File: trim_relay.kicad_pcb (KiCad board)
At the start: 2 copper layers, 75 x 75 mm, 45 parts, among them J1 Conn_01x01, J10 Conn_01x01, J11 Conn_01x01, J2 Conn_01x01, J3 Conn_01x01, J4 Conn_01x01, J5 Conn_01x01, J6 Conn_01x01, J7 Conn_01x01, J8 Conn_01x01, J9 Conn_01x01, K1 G5LE, K2 G5LE, K3 G5LE, K4 G5LE, K5 G5LE, Q1 2N3906, Q2 2N3906, Q3 2N3906, Q4 2N3906, Q5 2N3906, U1 LM317L_TO92

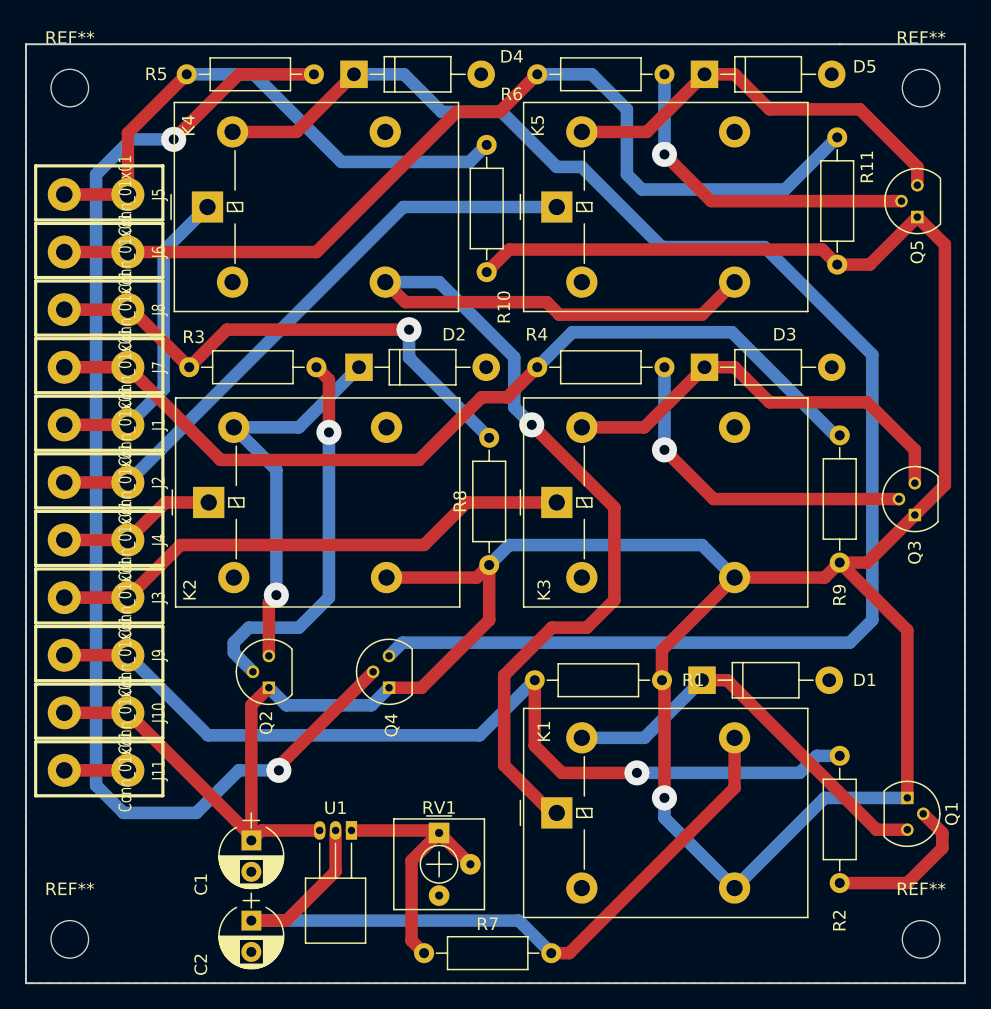
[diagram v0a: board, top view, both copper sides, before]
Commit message: Fixed layout
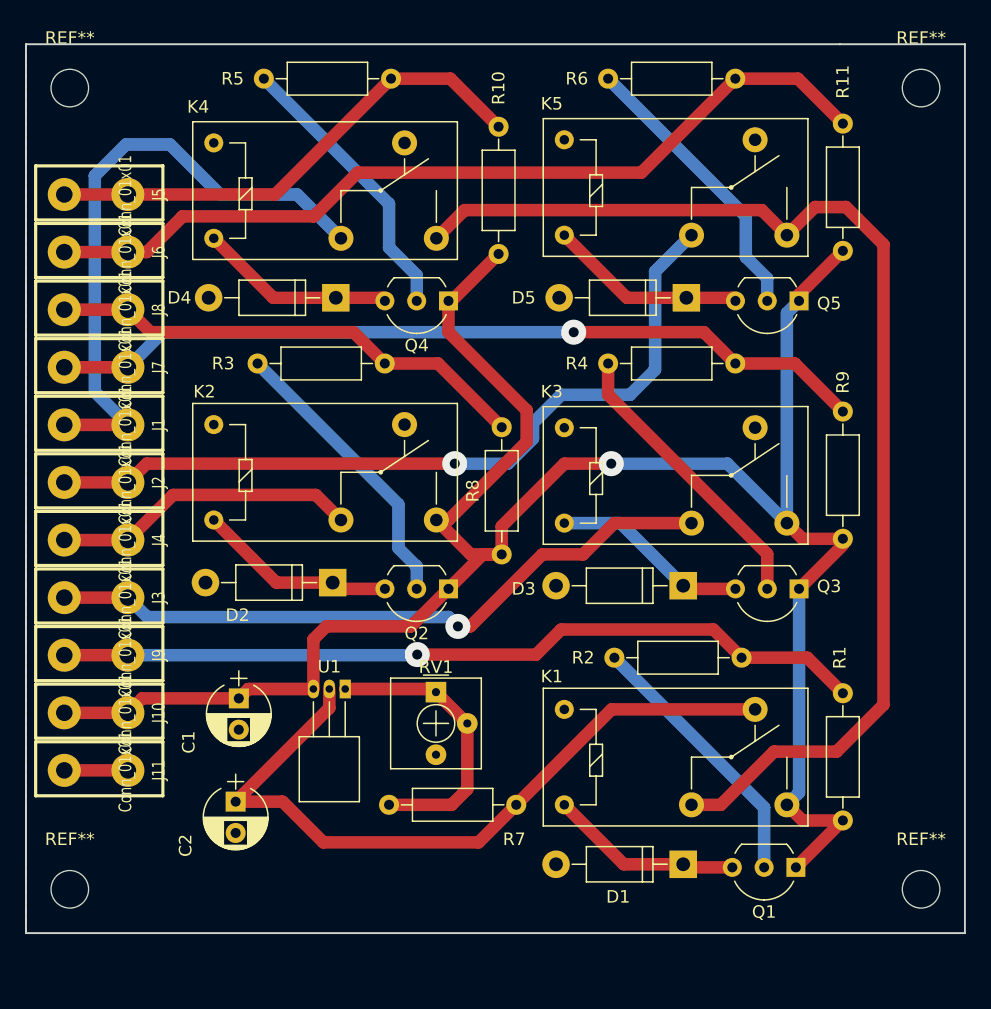
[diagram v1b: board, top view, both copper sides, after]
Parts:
- C1, C2: value CP -> 0.68uF
- K1, K2, K3, K4, K5: value G5LE -> G5Q-14 DC12; footprint Relays_THT:Relay_SPDT_OMRON-G5LE-1 -> Relays_THT:Relay_SPDT_OMRON-G5Q
- Q1, Q2, Q3, Q4, Q5: footprint TO_SOT_Packages_THT:TO-92_Molded_Narrow -> TO_SOT_Packages_THT:TO-92_Inline_Wide
- R1, R10, R11, R8, R9: value R -> 10K
- R2, R3, R4, R5, R6: value R -> 3K9
- R7: value R -> 120
- RV1: value POT -> 1K
- moved Q4 31.3 mm to (73.8, 60.5), turned to 180 degrees
- moved R2 25.5 mm to (87.0, 89.0), turned to 0 degrees
- moved R1 18.3 mm to (105.2, 102.0), turned to 90 degrees
- moved D4 17.9 mm to (64.8, 60.2), turned to 180 degrees
- moved D5 17.9 mm to (92.8, 60.2), turned to 180 degrees
- moved D3 17.5 mm to (92.5, 83.2), turned to 180 degrees
- moved D2 17.3 mm to (64.5, 83.0), turned to 180 degrees
- moved Q2 16.4 mm to (73.8, 83.5), turned to 180 degrees
- moved D1 14.8 mm to (92.5, 105.5), turned to 180 degrees
- moved R7 12.2 mm to (69.0, 100.8)
- moved Q5 11.6 mm to (101.8, 60.5), turned to 180 degrees
- moved C1 11.4 mm to (57.0, 92.2)
- moved U1 11.3 mm to (65.5, 91.5)
- moved RV1 11.3 mm to (72.8, 91.8)
- moved Q3 11.0 mm to (101.8, 83.5), turned to 180 degrees
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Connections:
- K1 pad 1: V_ELEV -> Net-(D1-Pad1)
- K1 pad 2: GND -> V_ELEV
- K1 pad 5: Net-(D1-Pad1) -> GND
- K2 pad 1: TRIM_AL_UP_OUT -> Net-(D2-Pad1)
- K2 pad 2: GND -> TRIM_AL_UP_OUT
- K2 pad 5: Net-(D2-Pad1) -> GND
- K3 pad 1: TRIM_AL_DN_OUT -> Net-(D3-Pad1)
- K3 pad 2: GND -> TRIM_AL_DN_OUT
- K3 pad 5: Net-(D3-Pad1) -> GND
- K4 pad 1: TRIM_ELEV_UP_OUT -> Net-(D4-Pad1)
- K4 pad 2: GND -> TRIM_ELEV_UP_OUT
- K4 pad 5: Net-(D4-Pad1) -> GND
- K5 pad 1: TRIM_ELEV_DN_OUT -> Net-(D5-Pad1)
- K5 pad 2: GND -> TRIM_ELEV_DN_OUT
- K5 pad 5: Net-(D5-Pad1) -> GND
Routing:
- net Net-(D4-Pad1): track 123.3 -> 15.7 mm
- net Net-(Q4-Pad2): track 97.4 -> 22.8 mm, vias 2 -> 0
- net +12V: track 240.1 -> 169.1 mm
- net TRIM_ELEV_UP_OUT: track 25.1 -> 49.9 mm
- net Net-(D3-Pad1): track 34.0 -> 15.8 mm
- net Net-(D5-Pad1): track 33.2 -> 15.8 mm
- net Net-(D1-Pad1): track 32.9 -> 15.5 mm
- net Net-(D2-Pad1): track 31.9 -> 15.9 mm, vias 1 -> 0
- net TRIM_ELEV_DN_OUT: track 48.5 -> 63.6 mm, vias 0 -> 1
- net TRIM_AL_DN_OUT: track 42.5 -> 54.5 mm, vias 0 -> 1
- net TRIM_AL_UP_OUT: track 12.8 -> 24.4 mm
- net Net-(Q1-Pad2): track 12.7 -> 21.7 mm
- net FLAP_DN: track 73.1 -> 65.1 mm
- net Net-(Q2-Pad2): track 30.9 -> 23.3 mm, vias 1 -> 0
- net TRIM_ELEV_DN_IN: track 76.2 -> 69.4 mm
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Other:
- board size 75 x 75 mm -> 75 x 71 mm
- board text added: "www-bit-builder.com-trim_relay-v1.0"
